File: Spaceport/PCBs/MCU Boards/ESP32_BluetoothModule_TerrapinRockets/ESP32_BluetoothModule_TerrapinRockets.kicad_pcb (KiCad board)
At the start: 2 copper layers, 50.5 x 58 mm, 15 parts, among them J1 Conn_01x06, J3 Conn_01x06, U1 ESP32-WROOM-32D

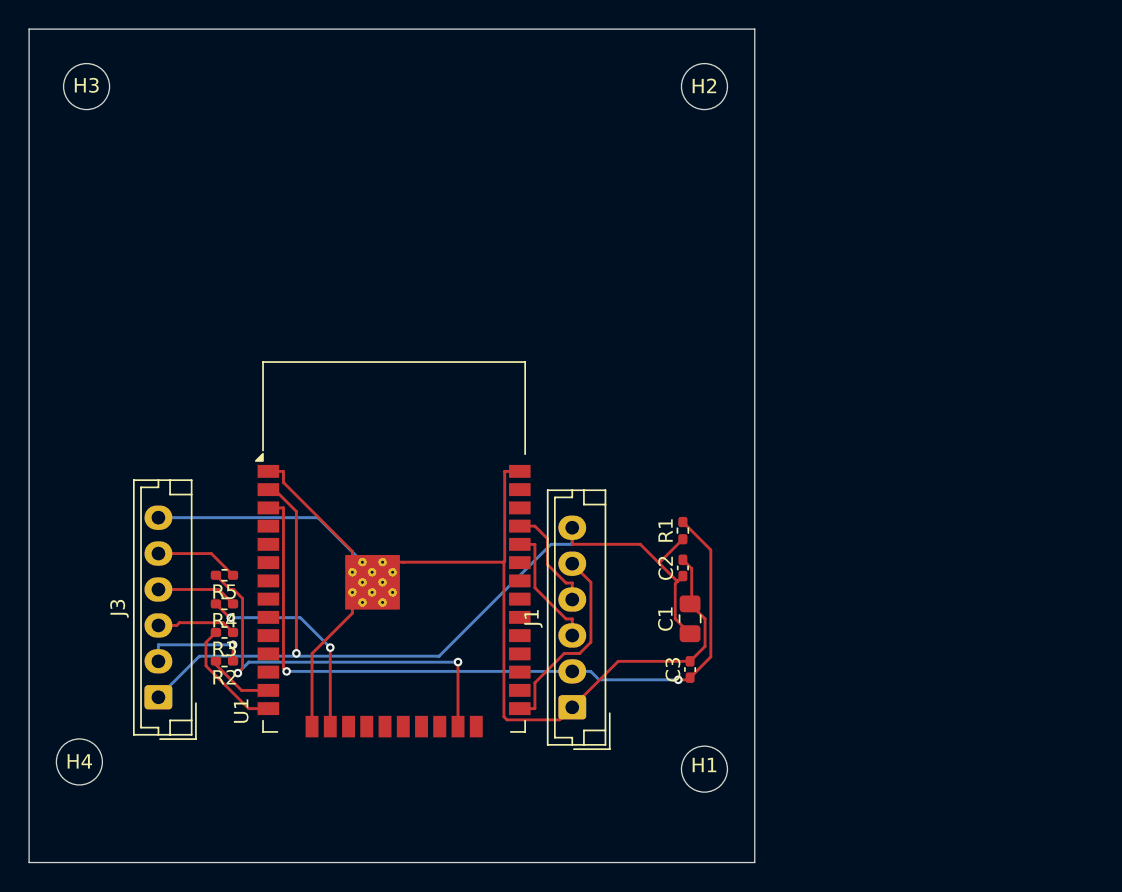
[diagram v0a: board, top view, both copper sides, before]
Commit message: modified schematic
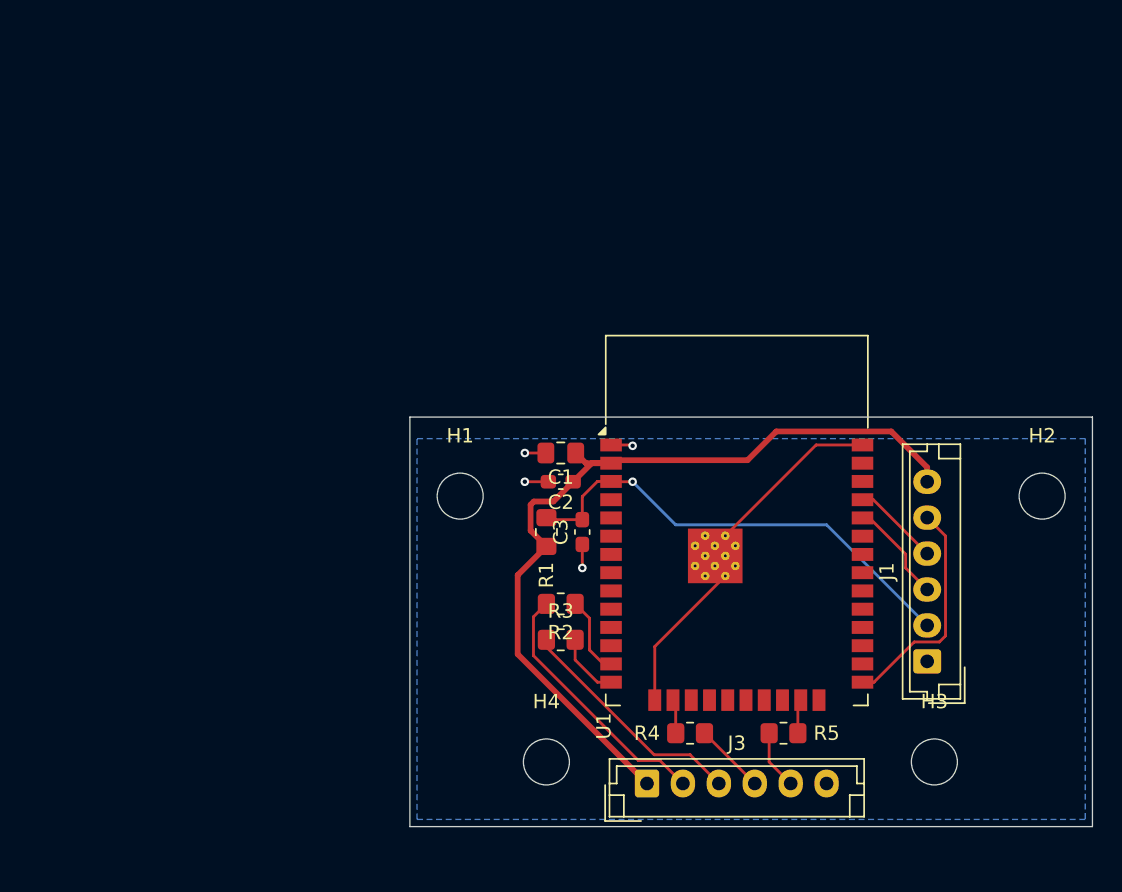
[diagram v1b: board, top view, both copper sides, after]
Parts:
- C2, C3: footprint Capacitor_SMD:C_0402_1005Metric_Pad0.74x0.62mm_HandSolder -> Capacitor_SMD:C_0603_1608Metric_Pad1.08x0.95mm_HandSolder
- R1, R2, R3, R4, R5: footprint Resistor_SMD:R_0402_1005Metric_Pad0.72x0.64mm_HandSolder -> Resistor_SMD:R_0805_2012Metric_Pad1.20x1.40mm_HandSolder
- moved H3 75.4 mm to (133.0, 129.0)
- moved R5 40.4 mm to (122.5, 127.0), turned to 0 degrees
- moved H2 36.9 mm to (140.5, 110.5)
- moved J3 34.5 mm to (113.0, 130.5), turned to 0 degrees
- moved R4 33.6 mm to (116.0, 127.0)
- moved H4 32.5 mm to (106.0, 129.0)
- moved H1 25.5 mm to (100.0, 110.5)
- moved J1 24.9 mm to (132.5, 122.0)
- moved U1 23.9 mm to (119.2, 115.2)
- moved R2 23.7 mm to (107.0, 118.0), turned to 0 degrees
- moved R3 23.4 mm to (107.0, 120.5), turned to 0 degrees
- moved C1 14.6 mm to (107.0, 107.5), turned to 180 degrees
- moved C3 12.2 mm to (108.5, 113.0), turned to -90 degrees
- moved C2 10.4 mm to (107.0, 109.5), turned to 180 degrees
- moved R1 9.50 mm to (106.0, 113.0)
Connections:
- J1 pad 3: /TX -> /RX
- J1 pad 4: /RX -> /TX
- U1 pad 34: /TX -> /RX
- U1 pad 35: /RX -> /TX
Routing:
- net GND: track 102.6 -> 29.1 mm, vias 0 -> 4
- net Net-(U1-IO15): track 28.0 -> 2.38 mm, vias 2 -> 0
- net /EN: track 53.1 -> 32.7 mm, vias 2 -> 1
- net Net-(U1-IO13): track 14.7 -> 2.38 mm, vias 2 -> 0
- net Net-(J3-Pin_3): track 5.55 -> 16.4 mm
- net Net-(J3-Pin_2): track 7.48 -> 18.1 mm, vias 1 -> 0
- net +3.3V: track 63.6 -> 58.9 mm, vias 1 -> 0
- net Net-(U1-IO12): track 8.18 -> 4.54 mm
- net /TX: track 8.72 -> 6.05 mm
- net /IO0: track 13.9 -> 15.9 mm
- net Net-(J3-Pin_5): track 5.82 -> 4.12 mm
- net Net-(U1-IO14): track 4.64 -> 5.53 mm
- net Net-(J3-Pin_4): track 5.61 -> 4.95 mm
- added copper zone on B.Cu, net GND
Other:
- board size 50.5 x 58 mm -> 47.5 x 28.5 mm
